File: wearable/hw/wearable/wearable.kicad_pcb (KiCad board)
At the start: 2 copper layers, 102 parts, among them IC1 LM4041CILPR, J1 Data, J2 Conn_02x05_Odd_Even, J3 Interrupts, J4 Data, J5 Data, J8 USBC Charger, SW1 SW_Toggle, U1 LT3042xMSE, U2 BNO080, U3 nRF54L15-QFXX, U4 MAX77659AENV+, U5 ADS1299IPAG, Y1 32MHz, Y2 32.768kHz, Y3 32.768kHz

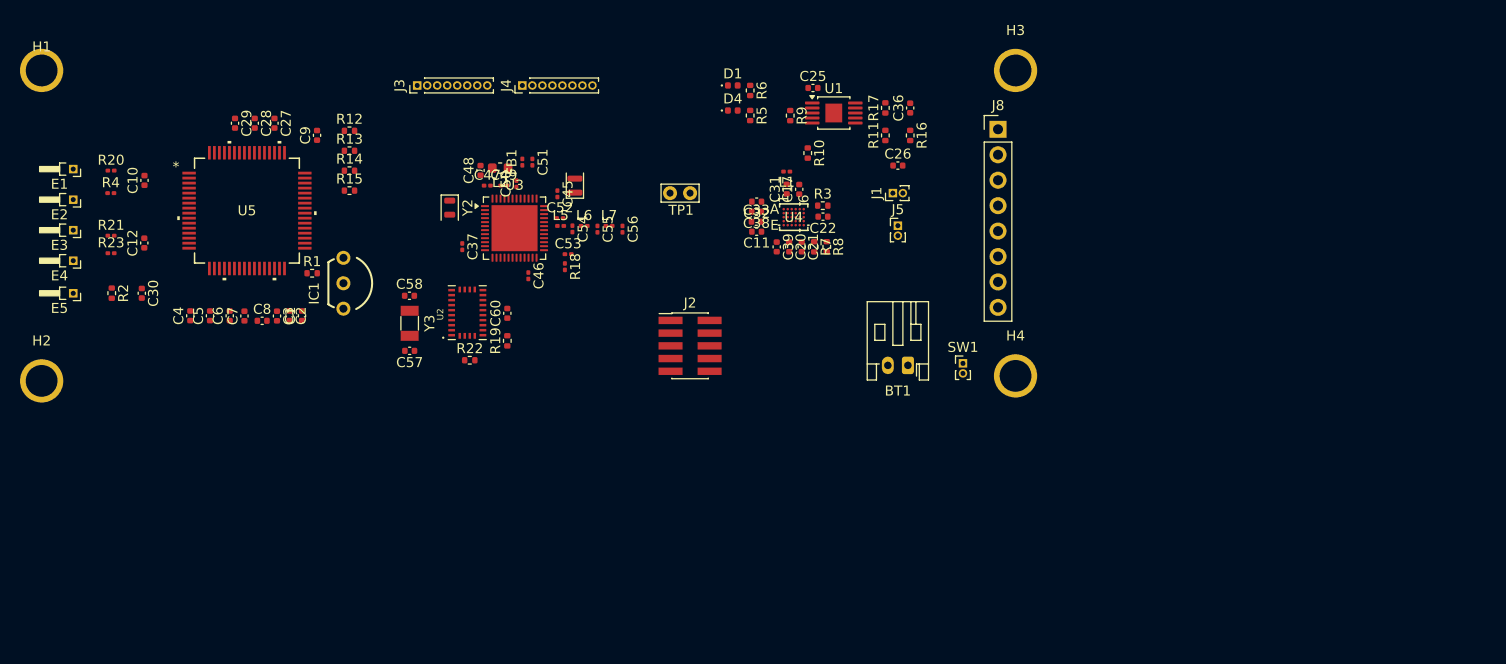
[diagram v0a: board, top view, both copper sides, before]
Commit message: Getting there
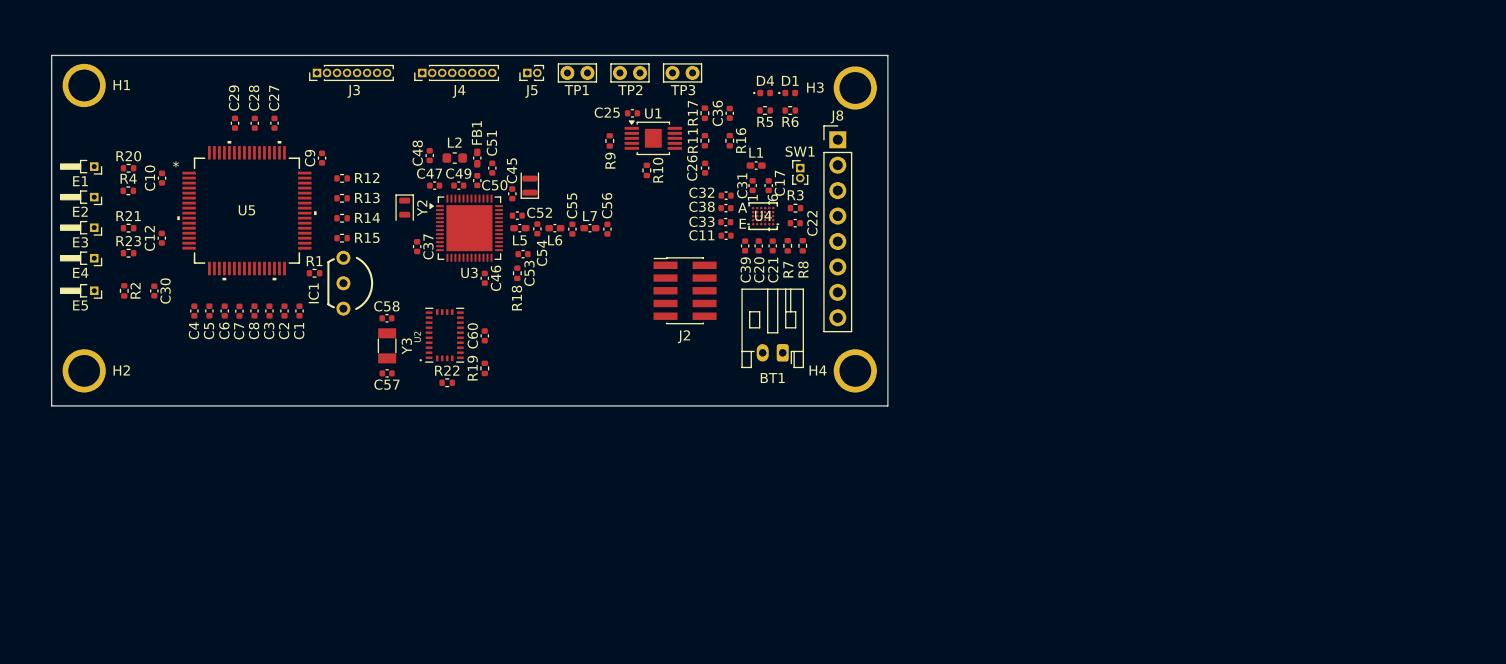
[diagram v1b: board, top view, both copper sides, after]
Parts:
- removed J1: Data, Connector_PinHeader_1.00mm:PinHeader_1x02_P1.00mm_Vertical
- added TP2: AVSS, TestPoint:TestPoint_Bridge_Pitch2.0mm_Drill0.7mm, F.Cu at (103.8, 62.8)
- added TP3: AVDD, TestPoint:TestPoint_Bridge_Pitch2.0mm_Drill0.7mm, F.Cu at (109.0, 62.8)
- C37, C45, C46, C47, C49, C50, C51, C52, C53, C54, C55, C56: footprint Capacitor_SMD:C_0201_0603Metric -> Capacitor_SMD:C_0402_1005Metric
- FB1, L5, L6, L7: footprint Inductor_SMD:L_0201_0603Metric -> Inductor_SMD:L_0402_1005Metric_Pad0.77x0.64mm_HandSolder
- L1: footprint Capacitor_SMD:C_0201_0603Metric -> Inductor_SMD:L_0402_1005Metric_Pad0.77x0.64mm_HandSolder
- R18, R20, R21, R23, R4: footprint Resistor_SMD:R_0201_0603Metric -> Resistor_SMD:R_0402_1005Metric
- moved J5 40.0 mm to (94.5, 62.8), turned to 90 degrees
- moved SW1 25.4 mm to (121.8, 72.2)
- moved C26 19.3 mm to (112.2, 72.2), turned to -90 degrees
- moved C25 18.2 mm to (105.0, 66.8)
- moved R9 18.2 mm to (102.7, 69.5)
- moved U1 18.2 mm to (107.1, 69.3)
- moved C36 18.0 mm to (114.7, 66.8)
- moved R11 18.0 mm to (112.2, 69.5)
- moved R16 18.0 mm to (114.7, 69.5)
- moved R17 18.0 mm to (112.2, 66.8)
- moved R10 16.2 mm to (106.4, 72.5)
- moved H3 16.1 mm to (127.2, 64.2)
- moved J8 16.0 mm to (125.5, 69.4)
- moved H4 16.0 mm to (127.2, 92.5)
- moved TP1 15.8 mm to (98.5, 62.8)
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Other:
- board outline added: 83.5 x 35 mm

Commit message: More layout progress and some fun stuff
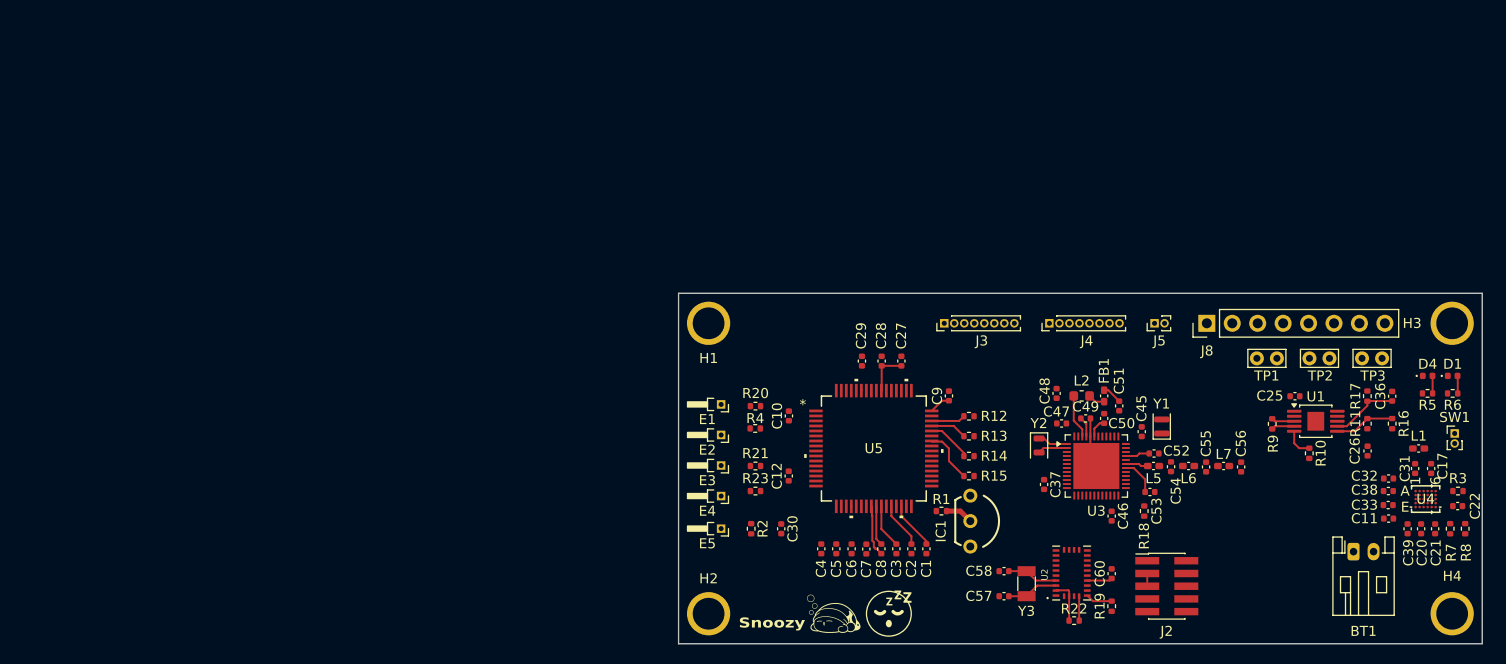
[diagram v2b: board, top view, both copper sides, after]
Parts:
- added G***: LOGO, LOGO, F.Cu at (130.6, 116.8)
- added G***: LOGO, LOGO, F.Cu at (125.1, 116.8)
- TP1: value BatteryStatus -> AVDD
- TP3: value AVDD -> BatteryStatus
- moved TP1 74.5 mm to (167.3, 91.2)
- moved TP2 74.5 mm to (172.6, 91.2)
- moved TP3 74.5 mm to (177.8, 91.2)
- moved C11 71.9 mm to (180.5, 107.2)
- moved C17 71.9 mm to (184.8, 102.2)
- moved C20 71.9 mm to (183.8, 108.3)
- moved C21 71.9 mm to (185.2, 108.3)
- moved C22 71.9 mm to (187.4, 106.0)
- moved C25 71.9 mm to (171.2, 95.0)
- moved C26 71.9 mm to (178.4, 100.5)
- moved C31 71.9 mm to (183.2, 102.2)
- moved C32 71.9 mm to (180.5, 103.2)
- moved C33 71.9 mm to (180.5, 105.9)
- moved C36 71.9 mm to (180.9, 95.0)
- moved C39 71.9 mm to (182.4, 108.3)
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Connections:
- TP1 pad 1: AMUX -> AVDD
- TP3 pad 1: AVDD -> AMUX
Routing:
- net Net-(U5-VREFP): track 0.00 -> 8.01 mm
- net AVSS: track 0.00 -> 6.88 mm
- net Net-(U1-SET): track 0.00 -> 6.78 mm
- net +3V3: track 0.00 -> 6.45 mm
- net Net-(U3-DECA): track 0.00 -> 6.37 mm
- net Net-(U1-PGFB): track 0.00 -> 6.01 mm
- net Net-(U5-GPIO1): track 0.00 -> 5.40 mm
- net /XIN: track 0.00 -> 5.15 mm
- net /XOUT: track 0.00 -> 5.10 mm
- net Net-(U5-VCAP2): track 0.00 -> 4.80 mm
- net Net-(U5-VCAP1): track 0.00 -> 4.59 mm
- net Net-(U5-VCAP3): track 0.00 -> 4.45 mm
- net Net-(U5-GPIO2): track 0.00 -> 4.44 mm
- net Net-(U3-DCC): track 0.00 -> 4.41 mm
- net Net-(U5-VCAP4): track 0.00 -> 4.38 mm
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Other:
- board size 83.5 x 35 mm -> 80.2 x 35 mm
- board text added: "ECE 464K: Aidan Aalund, Justin Bahn, Alex Ho, Kien Ton"
- board text added: "Snoozy"
